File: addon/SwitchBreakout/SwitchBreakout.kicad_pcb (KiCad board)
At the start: 2 copper layers, 127.8 x 194.6 mm, 209 parts, among them IC1 SN74HCS72QPWRQ1, IC10 SN74HCS72QPWRQ1, IC11 SN74HCS72QPWRQ1, IC12 SN74HCS72QPWRQ1, IC13 SN74HCS72QPWRQ1, IC14 SN74HCS72QPWRQ1, IC15 SN74HCS72QPWRQ1, IC16 SN74HCS72QPWRQ1, IC2 SN74HCS72QPWRQ1, IC3 SN74HCS72QPWRQ1, IC4 SN74HCS72QPWRQ1, IC5 SN74HCS72QPWRQ1, IC6 SN74HCS72QPWRQ1, IC7 SN74HCS72QPWRQ1, IC8 SN74HCS72QPWRQ1, IC9 SN74HCS72QPWRQ1, J1 SS73100-047F, J2 Conn_02x20_Odd_Even, J3 Conn_02x20_Odd_Even, J6 SS73100-047F, J7 SS73100-047F

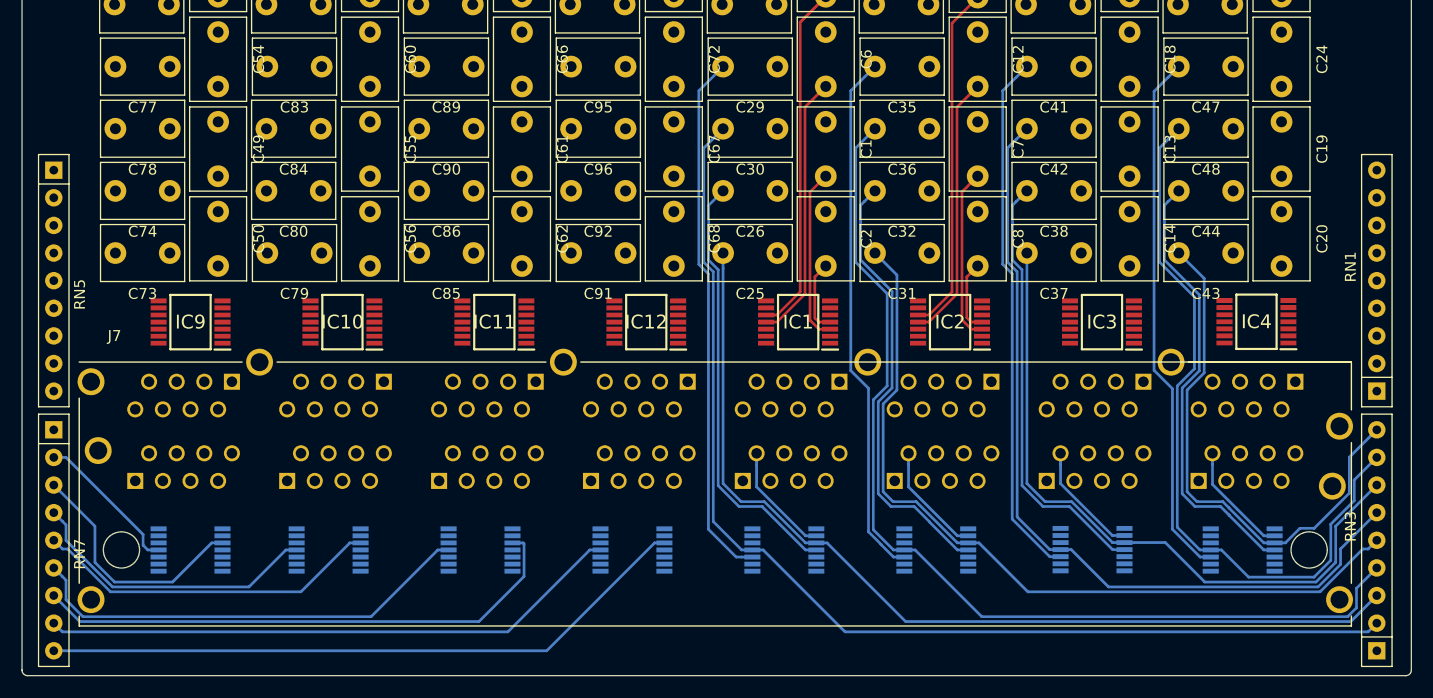
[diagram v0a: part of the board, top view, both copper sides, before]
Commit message: Swirls
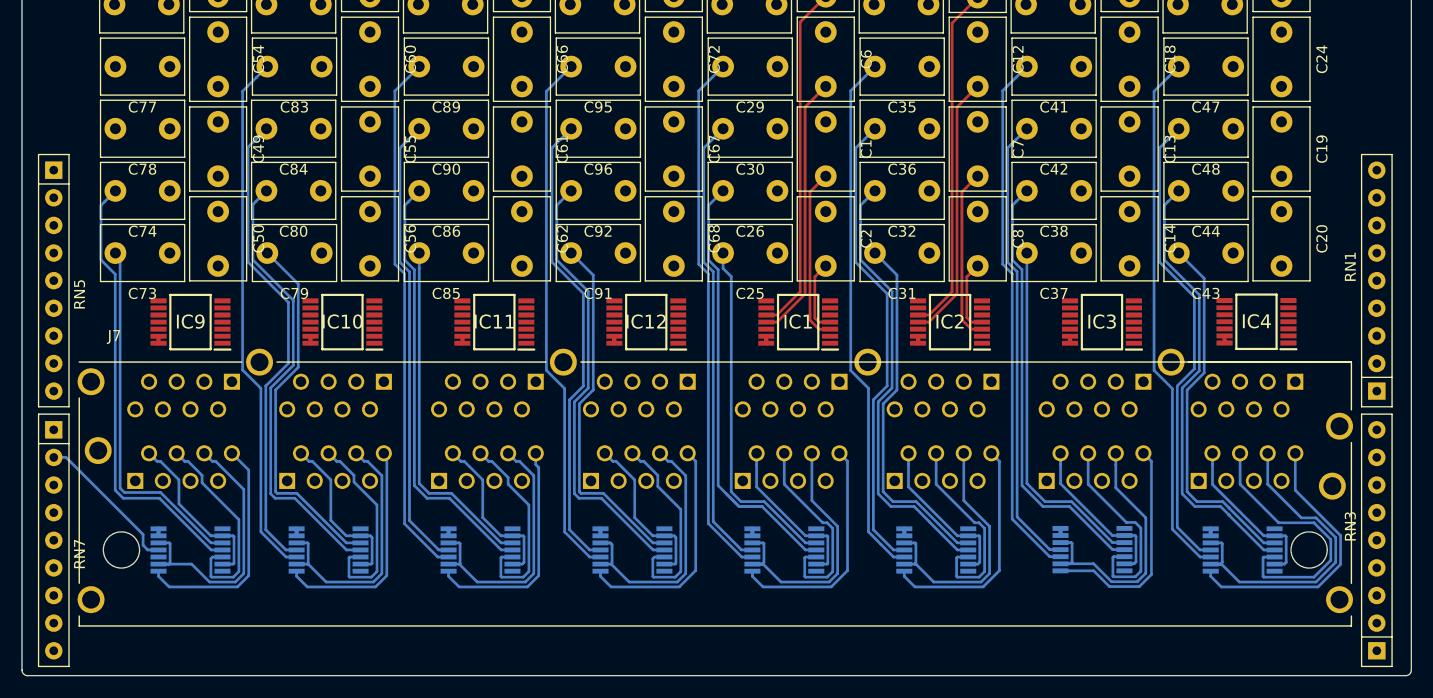
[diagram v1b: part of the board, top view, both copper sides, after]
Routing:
- net /D-Lach 9-16/D-Latch 0/CLK2: track 102.8 -> 41.9 mm
- net /D-Lach 9-16/D-Latch 0/CLK1: track 87.6 -> 32.0 mm
- net /D-Lach 9-16/D-Latch 1/CLK2: track 91.9 -> 43.0 mm
- net /D-Latch 25-32/D-Latch 4/BTN2: track 0.00 -> 48.7 mm
- net /D-Latch 25-32/D-Latch 1/BTN2: track 0.00 -> 48.7 mm
- net /D-Latch 25-32/D-Latch 2/BTN2: track 0.00 -> 48.7 mm
- net /D-Lach 9-16/D-Latch 1/CLK1: track 74.5 -> 33.1 mm
- net /D-Latch 25-32/D-Latch 1/BTN1: track 0.00 -> 41.2 mm
- net /D-Latch 25-32/D-Latch 0/BTN1: track 0.00 -> 40.8 mm
- net /D-Latch 25-32/D-Latch 4/BTN1: track 0.00 -> 40.5 mm
- net /D-Latch 25-32/D-Latch 2/BTN1: track 0.00 -> 39.5 mm
- net /D-Lach 9-16/D-Latch 2/CLK2: track 76.2 -> 42.0 mm
- net /D-Lach 9-16/D-Latch 2/CLK1: track 62.8 -> 32.4 mm
- net /A6: track 0.00 -> 30.3 mm
- net /D-Latch 25-32/D-Latch 4/CLK1: track 60.3 -> 33.1 mm
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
